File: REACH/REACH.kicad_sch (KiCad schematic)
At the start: 24 parts, among them J1 PACK, J2 FC-1, J3 PACK, J4 THERMOSTAT, J5 PACK, J6 FC-1, J7 THERMOSTAT, J8 PACK, J9 THERMOSTAT, U1 R1, U2 R2, U3 R1, U4 R2, U5 R1, U6 R2, U7 R1, U8 R2

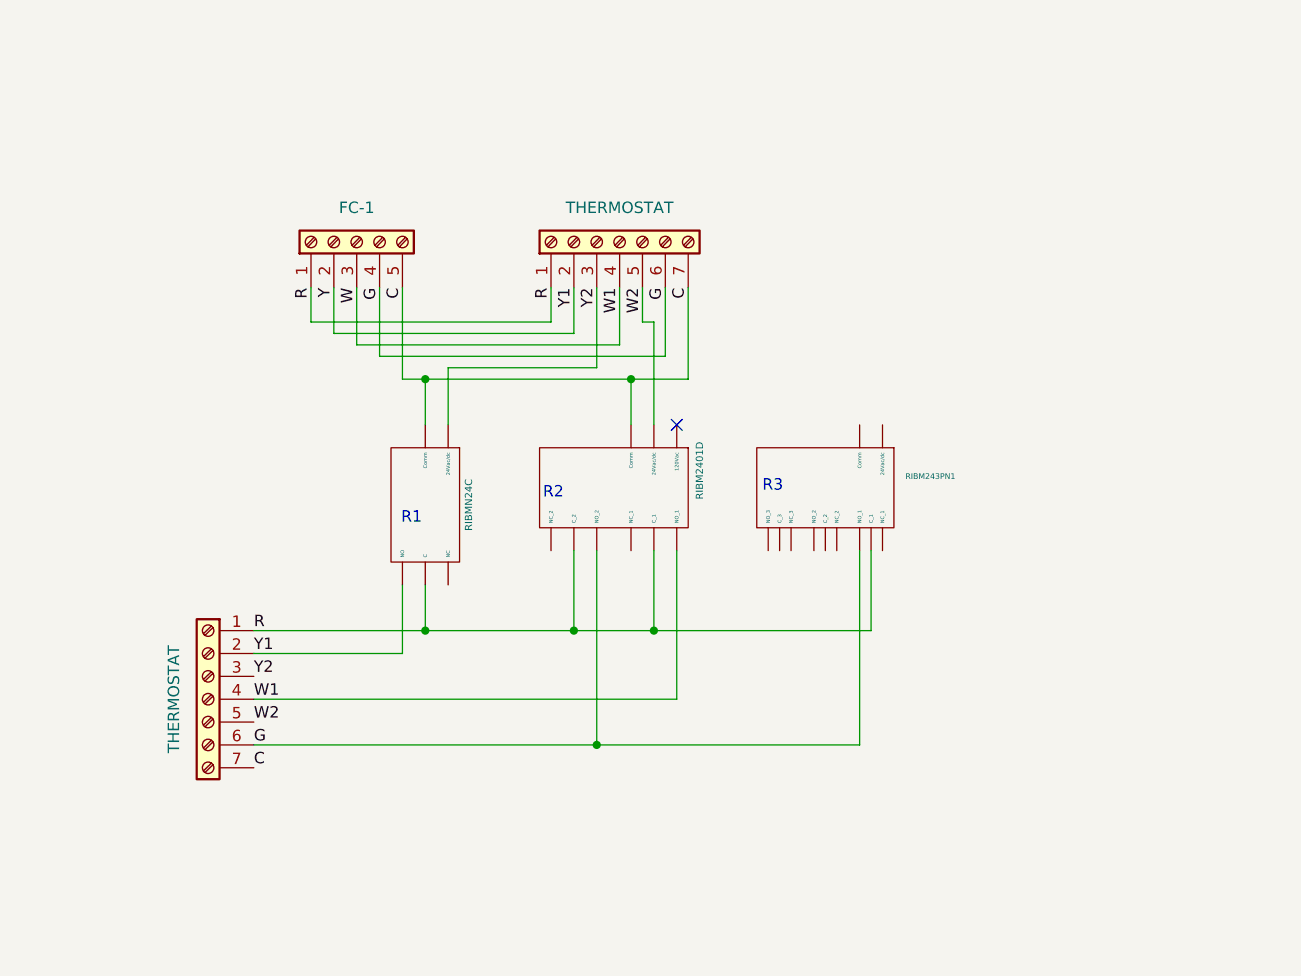
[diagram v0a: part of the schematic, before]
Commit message: .
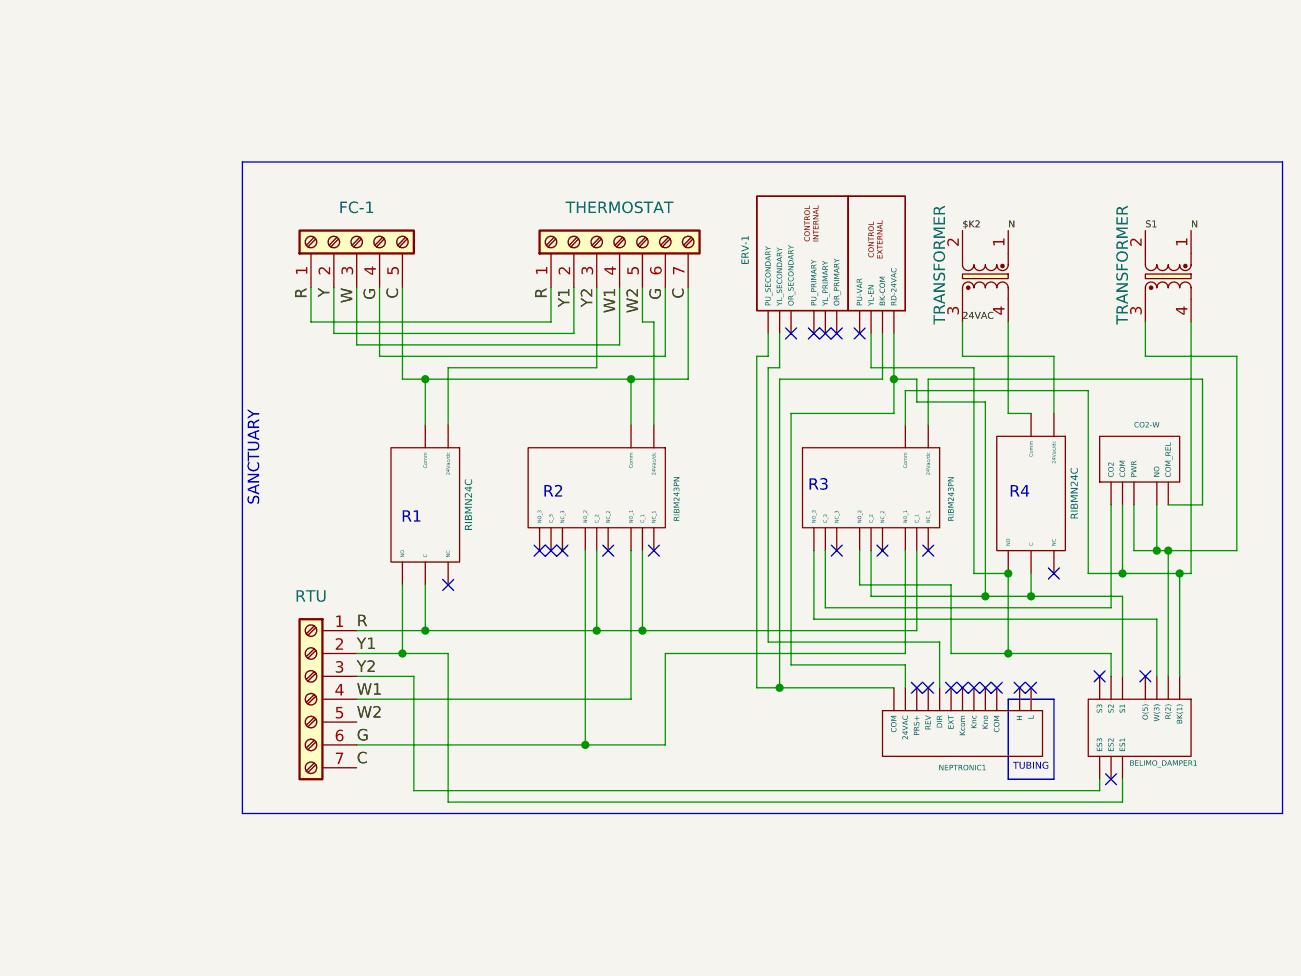
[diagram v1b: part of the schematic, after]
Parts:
- removed RIBM2401D: ~, symbol MYLIB:RIBM2401D
- added BELIMO_DAMPER1: ~, symbol lucasLib:BELIMO_DAMPER
- added CO2-W: ~, symbol lucasLib:CO2-W
- added ERV-1: ~, symbol lucasLib:ERV-1
- added NEPTRONIC1: ~, symbol lucasLib:NEPTRONIC
- added RIBM243PN: ~, symbol MYLIB:RIBM243PN
- added RIBMN24C: ~, symbol MYLIB:RIBMN24C
- added TR5, TR6: TRANSFORMER, Transformer_THT:Transformer_Zeming_ZMPT101K, symbol Transformer:ZMPT101K
- J9: value THERMOSTAT -> RTU
- renumbered RIBM243PN1 to RIBM243PN
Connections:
- net C: now also RIBM243PN. (NO_3)
- net G: now also RIBM243PN. (NO_3)
- net R: now also RIBM243PN. (NO_3)
- net W: now also RIBM243PN. (NO_3)
- net W2: now also RIBM243PN. (NO_3)
- net Y: now also BELIMO_DAMPER1. (ES3)
- net Y2: now also BELIMO_DAMPER1. (ES3)
- new net: U7. (WHT/Yel-Comm), U8. (WHT/Yel-Comm)
- new net: U5. (WHT/Yel-Comm), U7. (WHT/Yel-Comm)
- new net: U5. (WHT/Yel-Comm), U6. (WHT/Yel-Comm)
- new net: BELIMO_DAMPER1. (ES3), CO2-W. (COM_REL), TR6.3
- new net: BELIMO_DAMPER1. (ES3), CO2-W. (COM_REL), RIBM243PN. (NO_3), TR6.4
- new net: BELIMO_DAMPER1. (ES3), ERV-1. (PU_SECONDARY), NEPTRONIC1. (L), RIBM243PN. (NO_3), RIBMN24C. (NO)
- new net: BELIMO_DAMPER1. (ES3), ERV-1. (PU_SECONDARY), RIBM243PN. (NO_3), RIBMN24C. (NO)
- new net: BELIMO_DAMPER1. (ES3), RIBM243PN. (NO_3)
- new net: CO2-W. (COM_REL), RIBM243PN. (NO_3) (x2)
- new net: ERV-1. (PU_SECONDARY), NEPTRONIC1. (L) (x2)
- new net: RIBMN24C. (NO), TR5.4
- new net $K2: TR5.2
- new net 24VAC: RIBMN24C. (NO), TR5.3
- new net N: TR5.1, TR6.1
- new net S1: TR6.2
- no-connect marks 41 -> 67
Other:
- note added: "R4"
- note added: "SANCTUARY"
- note added: "TUBING"
- moved on the sheet: RIBM243PN
